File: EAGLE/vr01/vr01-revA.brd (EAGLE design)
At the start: 49.4 x 20 mm, 11 parts, among them J1 CX60-24S-UNIT, SW1 SPST_TACT-KMR2, SW2 SPST_TACT-KMR2, U1 ESP32-C6-MINI-1, U2 AP2112K-3.3

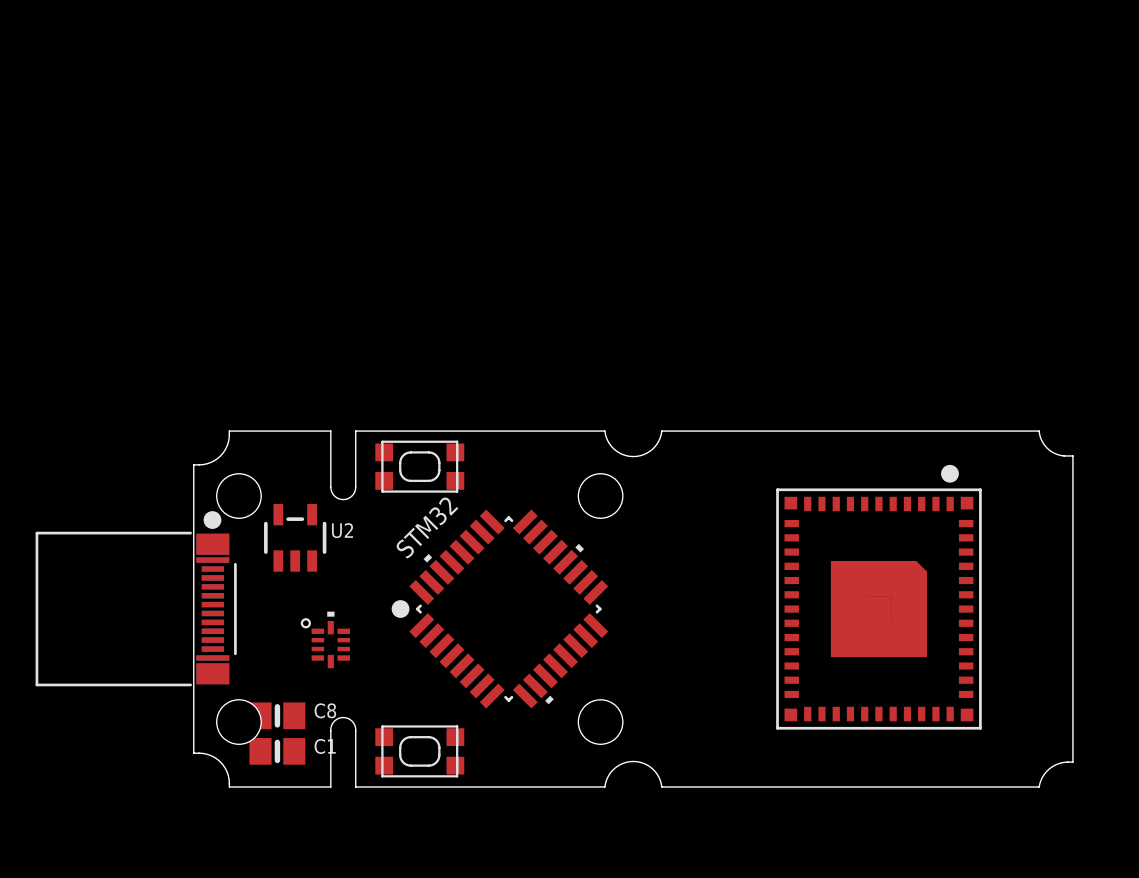
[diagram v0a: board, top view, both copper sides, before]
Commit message: .
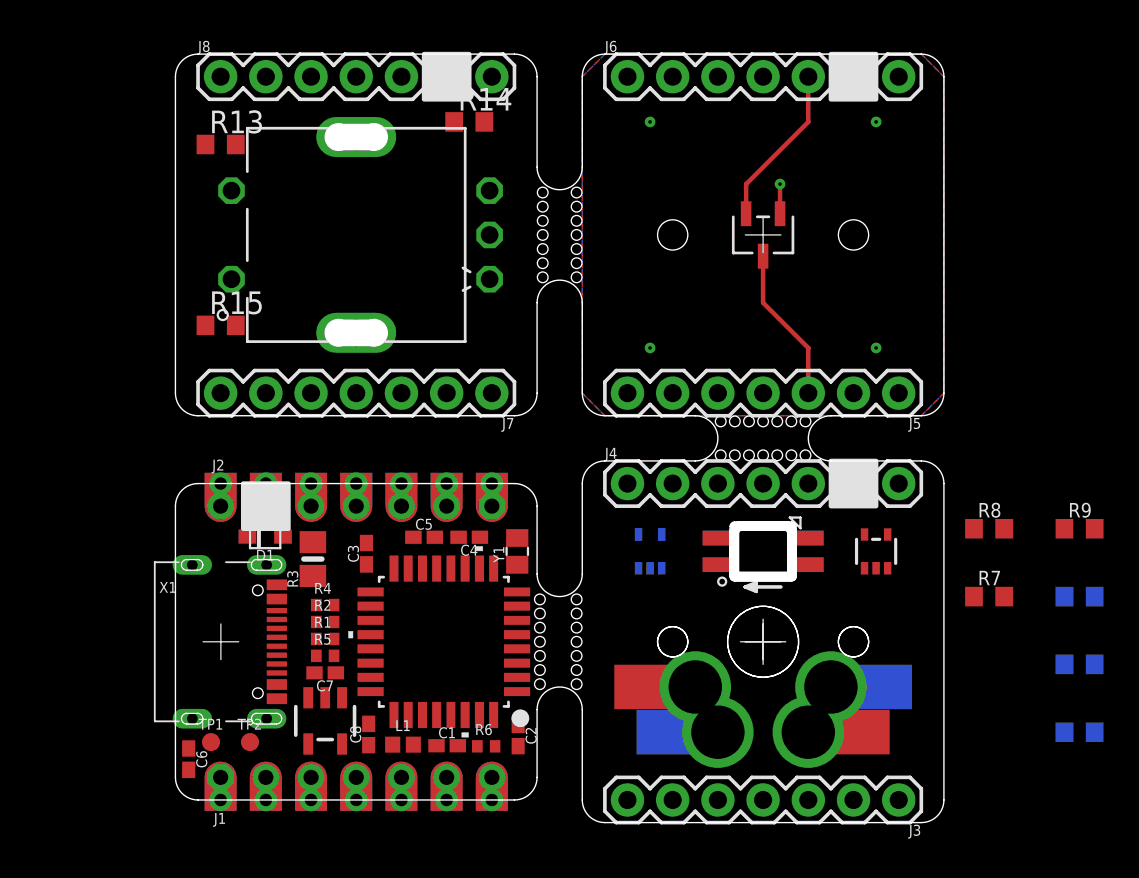
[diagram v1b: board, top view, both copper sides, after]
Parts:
- removed LK-USB07: CASE-LK-USB07-OPEN-ENDS, vr01-footprints:CASE-LK-USB07_OPEN_END
- removed SW1, SW2: SPST_TACT-KMR2, adafruit:KMR2
- removed U$3: TRINKEYDRILLS, __vr01-footprints:TRINKEY-DRILLS
- removed USBSEL: TS3USB221A-Q1, ts_kb_mcu:RSE10
- added C2, C3, C6: 100nF, rcl:C0402K
- added C4, C5: 4.3pF, rcl:C0402K
- added C7: 10uF, rcl:C0402K
- added D1: NSR0320, adafruit:SOD-323F
- added J2: (no value), Seeeduino-XIAO-footprint-eagle:H7-HALF-HOLE-2.54
- added J3, J4, J5, J6, J7, J8: (no value), SparkFun-Connectors:1X07
- added L1: BEAD, SparkFun-Coils:0402
- added R1, R2: 10R, rcl:R0402
- added R10, R15, R8: 10K, rcl:R0603
- added R11, R12, R7, R9: (no value), rcl:R0603
- added R13, R14: 5.1K, rcl:R0603
- added R3: FUSE, microbuilder:0805-NO
- added R4, R5: 5.1K, rcl:R0402
- added R6: 10K, rcl:R0402
- added TP1, TP2: TEST-POINT.4RN, tecsmith_keyboards:PAD.04X.04-RN
- added U$11, U$12: MX-5-PIN-HOTSWAP-VIANO-SILK, tecsmith_keyboards:MX-5-PIN-HOTSWAP-VIA-NS
- added U$13, U$14: SK6812-MINI-ESK6812MINI-E, tecsmith_keyboards:SK6812-E-MILL_V2
- added U$16, U$19: MX-FPRINT-100U-DOC, tecsmith_keyboards:MX-FPRINT-DOC-100U
- added U$17, U$18: 74AHCT1G125GW, tecsmith_keyboards:SOT353
- added U$21: HE-2-PIN-HOTSWAP, tecsmith_keyboards:HE-2-PIN-HOTSWAP-NS
- added X1: (no value), tecsmith_keyboards:TYPE-C-31-M-12
- added Y1: 3.2768KHz, OPL_Crystal Oscillator:X2-SMD-L2.0X1.2X0.55MM
- C1: value 10uF -> 100nF; device microbuilder:0805-NO -> rcl:C0402K
- C8: device microbuilder:0805-NO -> rcl:C0402K
- J1: value CX60-24S-UNIT -> (none); device vr01-footprints:CONN10_CX60-24S-UNIT_HIR -> Seeeduino-XIAO-footprint-eagle:H7-HALF-HOLE-2.54
- U1: value ESP32-C6-MINI-1 -> EC11E15244B2; device vr01-footprints:ESP32-C6_EXP -> tecsmith_keyboards:ROTARY_EC11E
- moved U1 36.1 mm to (11.4, 33.0), turned to 90 degrees
- moved J1 13.0 mm to (11.4, 2.54), turned to 90 degrees
- moved U2 10.4 mm to (9.68, 5.71), turned to 180 degrees
- moved C1 9.54 mm to (16.5, 4.32)
- moved C8 5.24 mm to (12.1, 4.95), turned to 90 degrees
- moved STM32 4.09 mm to (16.4, 10.2), turned to 180 degrees
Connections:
- removed net +3V3: C8.1, U2.5
- removed net +5V: C1.1, U2.1, U2.3
- removed net 3V3: U1.3
- removed net GND1: C1.2, C8.2, U2.2
- removed net GND2: USBSEL.5
- removed net USB1_N: USBSEL.2
- removed net USB1_P: USBSEL.1
- removed net USB2_N: USBSEL.4
- removed net USB2_P: USBSEL.3
- removed net VCC: USBSEL.10
- removed net VDD: STM32.1
- removed net VDDA: STM32.5
- removed net VDDIO2: STM32.17
- removed net VSS: STM32.16, STM32.32
- new net !RST: C6.1, STM32.4, TP1.1
- new net A0D0: J1.1, J1.13, STM32.6
- new net A1D1: J1.14, J1.2, STM32.7
- new net A2D2: J1.15, J1.3, STM32.8
- new net A3D3: J1.16, J1.4, STM32.9
- new net BOOT0: R6.2, STM32.31
- new net ENC1: J7.7, R13.1, U1.A
- new net ENC2: J8.1, R14.1, U1.B
- new net GND: C1.2, C2.2, C3.2, C4.2, C5.2, C6.2, C7.2, C8.2, J2.18, J2.6, J4.6, J6.6, J8.6, R10.1, R15.1, R4.2, R5.2, R6.1, R8.1, STM32.16, STM32.32, TP2.1, U$13.3-GND, U$14.3-GND, U$17.1, U$17.3, U$18.1, U$18.3, U$21.2, U1.C, U2.2, X1.A1B12-GND, X1.B1A12-GND, X1.M1, X1.M2, X1.M3, X1.M4
- new net HE1: J5.3, U$21.3
- new net LED: STM32.26
- new net MISO: J2.15, J2.3, STM32.12
- new net MOSI: J2.16, J2.4, STM32.13
- new net N$1: C1.1, L1.2, STM32.5
- new net N$10: R9.1, U$13.4-DIN
- new net N$11: R9.2, U$17.4
- new net N$12: R12.1, U$14.4-DIN
- new net N$13: R12.2, U$18.4
- new net N$14: R11.1, U$18.2
- new net N$15: R7.1, U$17.2
- new net N$2: C4.1, STM32.2, Y1.2
- new net N$3: C5.1, STM32.3, Y1.1
- new net N$4: R4.1, X1.A5-CC1
- new net N$5: R5.1, X1.B5-CC2
- new net N$6: C7.1, D1.C, U2.1, U2.3
- new net N$7: D1.A, R3.2
- new net N$8: R1.1, X1.A6-DP1, X1.B6-DP2
- new net N$9: R2.1, X1.A7-DN1, X1.B7-DN2
- new net NSS: STM32.10
- new net RCC: STM32.18
- new net RGB: J3.1, R11.2, R7.2
- new net RX: J2.1, J2.13, STM32.30
- new net SCK: J2.14, J2.2, STM32.11
- new net SCL: J1.18, J1.6, STM32.29
- new net SDA: J1.17, J1.5, STM32.20
- new net SW1: J3.4, R10.2, R8.2, U$11.2@1, U$11.2@2, U$12.1@1, U$12.1@2
- new net SW2: J7.2, R15.2, U1.E
- new net SWCLK: STM32.24
- new net SWDIO: STM32.23
- new net TX: J1.19, J1.7, STM32.19
- new net USB_N: R2.2, STM32.21
- new net USB_P: R1.2, STM32.22
- new net VCC3: C2.1, C3.1, C8.1, J2.17, J2.5, J4.5, J6.5, J8.5, L1.1, R13.2, R14.2, STM32.1, STM32.17, U$11.1@1, U$11.1@2, U$12.2@1, U$12.2@2, U$21.1, U1.D, U2.5
- new net VCC5: J2.19, J2.7, J4.7, J6.7, J8.7, R3.1, U$13.1-VDD, U$14.1-VDD, U$17.5, U$18.5, X1.A4B9-VBUS, X1.B4A9-VBUS
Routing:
- net VCC3: track 0.00 -> 9.14 mm
- net HE1: track 0.00 -> 8.75 mm
- net GND: track 0.00 -> 1.66 mm, vias 0 -> 5
- added copper zone on layer 1, net GND
- added copper zone on layer 15, net GND
- added copper zone on layer 16, net GND
- added copper zone on layer 2, net GND
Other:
- board size 49.4 x 20 mm -> 43.2 x 43.2 mm
- board text removed: "USE 0.8mm PCB ONLY"
